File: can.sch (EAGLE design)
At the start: 36 parts, among them IC1 LM1117IMP-5.0, J1 AVR_SPI_PRG_6NS, Q1 FDS5680, Q2 FDS5680, Q3 FDS5680, U1 ATMEGA8, U2 MCP2510SO, U3 MCP2551SN, U5 SG-8002CA

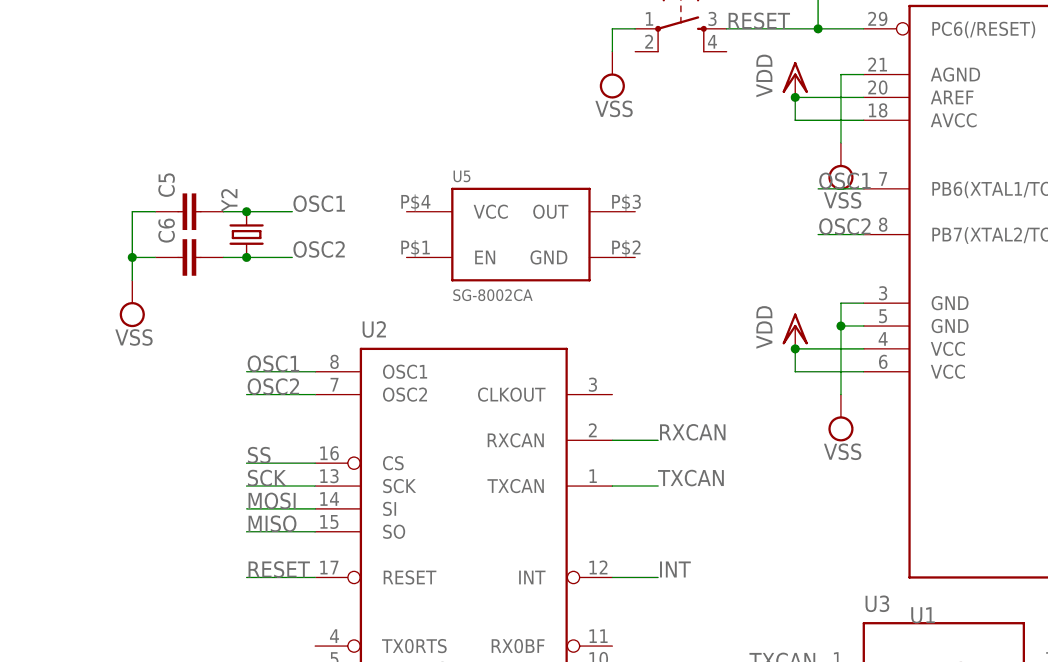
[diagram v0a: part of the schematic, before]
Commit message: 1.0.2
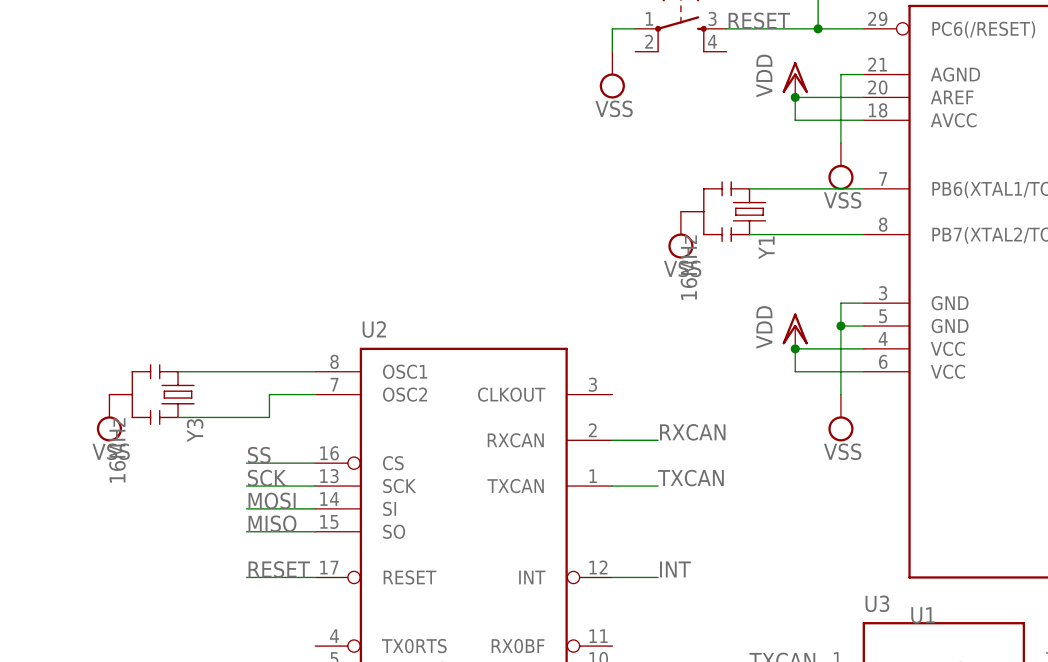
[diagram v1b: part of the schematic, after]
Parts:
- removed C5, C6: (no value), SparkFun-Capacitors:CAP1206
- removed U5: SG-8002CA, SparkFun-FreqCtrl:OSCILLATORSMD
- removed Y2: (no value), SparkFun-FreqCtrl:CRYSTALHC49US
- added Y1, Y3: 16MHz, SparkFun-FreqCtrl:RESONATOR16MHZ
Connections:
- removed net OSC1: C5.2, U1.PB6(XTAL1/TOSC1), U2>NAME.OSC1, Y2.2
- removed net OSC2: C6.2, U1.PB7(XTAL2/TOSC2), U2>NAME.OSC2, Y2.1
- new net N$12: U1.PB6(XTAL1/TOSC1), Y1.1
- new net N$14: U1.PB7(XTAL2/TOSC2), Y1.3
- new net N$16: U2>NAME.OSC1, Y3.1
- new net N$19: U2>NAME.OSC2, Y3.3
- net VSS: now also Y1.2, Y3.2; no longer C5.1, C6.1
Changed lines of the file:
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@@
 <part name="U2" library="microchip_can" deviceset="MCP2510" device="SO"/>
 <part name="U3" library="microchip_can" deviceset="MCP2551" device="SN"/>
-<part name="Y2" library="SparkFun-FreqCtrl" deviceset="CRYSTAL" device="HC49US"/>
-<part name="C5" library="SparkFun-Capacitors" deviceset="CAP" device="1206"/>
-<part name="C6" library="SparkFun-Capacitors" deviceset="CAP" device="1206"/>
 <part name="VDD1" library="supply1" deviceset="VDD" device=""/>
 <part name="VDD2" library="supply1" deviceset="VDD" device=""/>
@@
 <part name="SUPPLY3" library="supply2" deviceset="VSS" device=""/>
 <part name="SUPPLY5" library="supply2" deviceset="VSS" device=""/>
-<part name="SUPPLY6" library="supply2" deviceset="VSS" device=""/>
 <part name="SUPPLY8" library="supply2" deviceset="VSS" device=""/>
 <part name="SUPPLY9" library="supply2" deviceset="VSS" device=""/>
@@
 <part name="R11" library="SparkFun-Resistors" deviceset="RESISTOR" device="1206"/>
 <part name="R12" library="SparkFun-Resistors" deviceset="RESISTOR" device="1206"/>
-<part name="U5" library="SparkFun-FreqCtrl" deviceset="OSCILLATOR" device="SMD" value="SG-8002CA"/>
+<part name="Y1" library="SparkFun-FreqCtrl" deviceset="RESONATOR" device="16MHZ" value="16MHz"/>
+<part name="Y3" library="SparkFun-FreqCtrl" deviceset="RESONATOR" device="16MHZ" value="16MHz"/>
+<part name="SUPPLY21" library="supply2" deviceset="VSS" device=""/>
+<part name="SUPPLY6" library="supply2" deviceset="VSS" device=""/>
 </parts>
 <sheets>
@@
 <instance part="U2" gate="&gt;NAME" x="-50.8" y="30.48"/>
 <instance part="U3" gate="&gt;NAME" x="5.08" y="5.08"/>
-<instance part="Y2" gate="G$1" x="-73.66" y="58.42" rot="R90"/>
-<instance part="C5" gate="G$1" x="-78.74" y="60.96" rot="R90"/>
-<instance part="C6" gate="G$1" x="-78.74" y="55.88" rot="R90"/>
 <instance part="VDD1" gate="G$1" x="-12.7" y="76.2"/>
 <instance part="VDD2" gate="G$1" x="-12.7" y="48.26"/>
@@
 <instance part="SUPPLY3" gate="G$1" x="86.36" y="71.12"/>
 <instance part="SUPPLY5" gate="G$1" x="-30.48" y="-2.54"/>
-<instance part="SUPPLY6" gate="G$1" x="-86.36" y="50.8"/>
 <instance part="SUPPLY8" gate="G$1" x="-7.62" y="38.1"/>
 <instance part="SUPPLY9" gate="G$1" x="-33.02" y="76.2"/>
@@
 <instance part="R11" gate="G$1" x="81.28" y="63.5" rot="R180"/>
 <instance part="R12" gate="G$1" x="81.28" y="40.64" rot="R180"/>
-<instance part="U5" gate="G$1" x="-43.18" y="58.42"/>
+<instance part="Y1" gate="G$1" x="-17.78" y="60.96" rot="R270"/>
+<instance part="Y3" gate="G$1" x="-81.28" y="40.64" rot="R270"/>
+<instance part="SUPPLY21" gate="G$1" x="-88.9" y="38.1"/>
+<instance part="SUPPLY6" gate="G$1" x="-25.4" y="58.42"/>
 </instances>
 <busses>
@@
 </segment>
 </net>
-<net name="OSC1" class="0">
-<segment>
-<pinref part="C5" gate="G$1" pin="2"/>
-<pinref part="Y2" gate="G$1" pin="2"/>
-<wire x1="-76.2" y1="60.96" x2="-73.66" y2="60.96" width="0.1524" layer="91"/>
-<wire x1="-73.66" y1="60.96" x2="-68.58" y2="60.96" width="0.1524" layer="91"/>
-<label x="-68.58" y="60.96" size="1.778" layer="95"/>
-<junction x="-73.66" y="60.96"/>
-</segment>
-<segment>
-<pinref part="U1" gate="G$1" pin="PB6(XTAL1/TOSC1)"/>
-<wire x1="-5.08" y1="63.5" x2="-10.16" y2="63.5" width="0.1524" layer="91"/>
-<label x="-10.16" y="63.5" size="1.778" layer="95"/>
-</segment>
-<segment>
-<pinref part="U2" gate="&gt;NAME" pin="OSC1"/>
-<wire x1="-66.04" y1="43.18" x2="-73.66" y2="43.18" width="0.1524" layer="91"/>
-<label x="-73.66" y="43.18" size="1.778" layer="95"/>
-</segment>
-</net>
-<net name="OSC2" class="0">
-<segment>
-<pinref part="Y2" gate="G$1" pin="1"/>
-<pinref part="C6" gate="G$1" pin="2"/>
-<wire x1="-73.66" y1="55.88" x2="-76.2" y2="55.88" width="0.1524" layer="91"/>
-<wire x1="-73.66" y1="55.88" x2="-68.58" y2="55.88" width="0.1524" layer="91"/>
-<label x="-68.58" y="55.88" size="1.778" layer="95"/>
-<junction x="-73.66" y="55.88"/>
-</segment>
-<segment>
-<pinref part="U1" gate="G$1" pin="PB7(XTAL2/TOSC2)"/>
-<wire x1="-5.08" y1="58.42" x2="-10.16" y2="58.42" width="0.1524" layer="91"/>
-<label x="-10.16" y="58.42" size="1.778" layer="95"/>
-</segment>
-<segment>
-<pinref part="U2" gate="&gt;NAME" pin="OSC2"/>
-<wire x1="-66.04" y1="40.64" x2="-73.66" y2="40.64" width="0.1524" layer="91"/>
-<label x="-73.66" y="40.64" size="1.778" layer="95"/>
-</segment>
-</net>
 <net name="SS" class="0">
 <segment>
@@
 <pinref part="R2" gate="G$1" pin="2"/>
 <pinref part="SUPPLY3" gate="G$1" pin="VSS"/>
-</segment>
-<segment>
-<pinref part="C5" gate="G$1" pin="1"/>
-<wire x1="-83.82" y1="60.96" x2="-86.36" y2="60.96" width="0.1524" layer="91"/>
-<wire x1="-86.36" y1="60.96" x2="-86.36" y2="55.88" width="0.1524" layer="91"/>
-<pinref part="C6" gate="G$1" pin="1"/>
-<wire x1="-86.36" y1="55.88" x2="-86.36" y2="53.34" width="0.1524" layer="91"/>
-<wire x1="-83.82" y1="55.88" x2="-86.36" y2="55.88" width="0.1524" layer="91"/>
-<junction x="-86.36" y="55.88"/>
-<pinref part="SUPPLY6" gate="G$1" pin="VSS"/>
 </segment>
 <segment>
@@
 <pinref part="SUPPLY19" gate="G$1" pin="VSS"/>
 </segment>
+<segment>
+<pinref part="Y3" gate="G$1" pin="2"/>
+<pinref part="SUPPLY21" gate="G$1" pin="VSS"/>
+</segment>
+<segment>
+<pinref part="Y1" gate="G$1" pin="2"/>
+<pinref part="SUPPLY6" gate="G$1" pin="VSS"/>
+</segment>
 </net>
 <net name="N$7" class="0">
@@
 </segment>
 </net>
+<net name="N$12" class="0">
+<segment>
+<pinref part="U1" gate="G$1" pin="PB6(XTAL1/TOSC1)"/>
+<pinref part="Y1" gate="G$1" pin="1"/>
+<wire x1="-5.08" y1="63.5" x2="-17.78" y2="63.5" width="0.1524" layer="91"/>
+</segment>
+</net>
+<net name="N$14" class="0">
+<segment>
+<pinref part="U1" gate="G$1" pin="PB7(XTAL2/TOSC2)"/>
+<pinref part="Y1" gate="G$1" pin="3"/>
+<wire x1="-5.08" y1="58.42" x2="-17.78" y2="58.42" width="0.1524" layer="91"/>
+</segment>
+</net>
+<net name="N$16" class="0">
+<segment>
+<pinref part="U2" gate="&gt;NAME" pin="OSC1"/>
+<pinref part="Y3" gate="G$1" pin="1"/>
+<wire x1="-66.04" y1="43.18" x2="-81.28" y2="43.18" width="0.1524" layer="91"/>
+</segment>
+</net>
+<net name="N$19" class="0">
+<segment>
+<pinref part="U2" gate="&gt;NAME" pin="OSC2"/>
+<wire x1="-66.04" y1="40.64" x2="-71.12" y2="40.64" width="0.1524" layer="91"/>
+<wire x1="-71.12" y1="40.64" x2="-71.12" y2="38.1" width="0.1524" layer="91"/>
+<pinref part="Y3" gate="G$1" pin="3"/>
+<wire x1="-71.12" y1="38.1" x2="-81.28" y2="38.1" width="0.1524" layer="91"/>
+</segment>
+</net>
